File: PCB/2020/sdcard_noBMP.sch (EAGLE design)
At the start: 23 parts, among them J1 CONN_20X2NOSILK, J2 CONN_20X2NOSILK, J3 CONN_20X2NOSILK, J4 CONN_20X2NOSILK, X1 JST-XH-12-PIN-LONG-PAD, X2 JST-XH-06-PIN-LONG-PAD, X3 JST-XH-06-PIN-LONG-PAD, X4 JST-XH-12-PIN-LONG-PAD

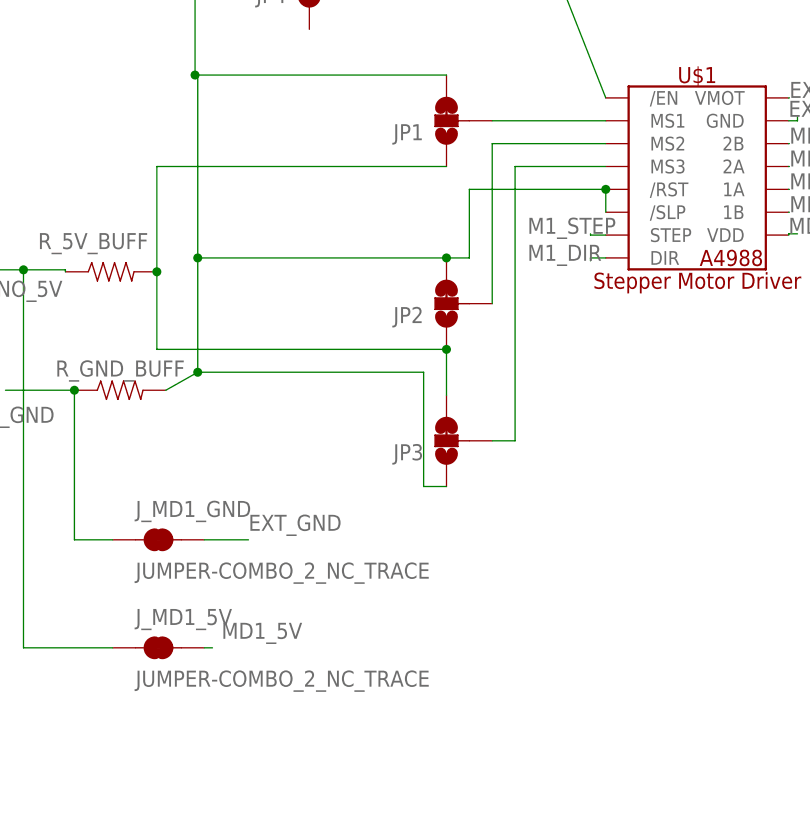
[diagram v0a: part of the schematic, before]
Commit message: PCB update
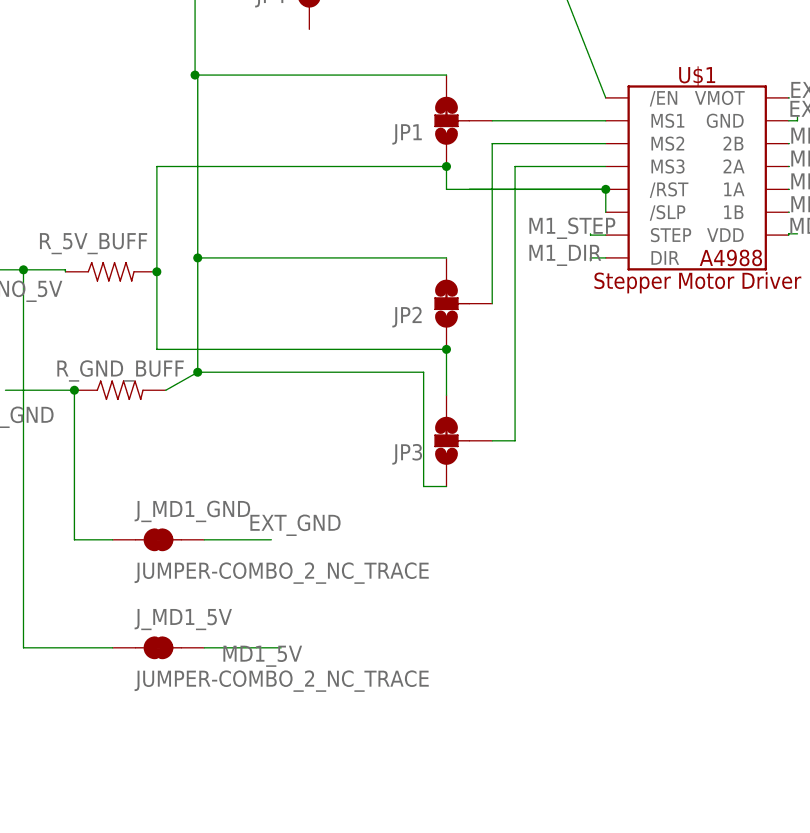
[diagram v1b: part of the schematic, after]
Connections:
- removed net N$9: JP1.1, JP2.1, JP3.3, R_5V_BUFF.2
- new net N$1: JP1.1, JP2.1, JP3.3, R_5V_BUFF.2, U$1./RST, U$1./SLP
- net N$14: no longer U$1./RST, U$1./SLP
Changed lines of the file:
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@@
 <?xml version="1.0" encoding="utf-8"?>
 <!DOCTYPE eagle SYSTEM "eagle.dtd">
-<eagle version="9.2.2">
+<eagle version="9.6.0">
 <drawing>
 <settings>
@@
 </segment>
 </net>
-<net name="N$9" class="0">
-<segment>
-<pinref part="R_5V_BUFF" gate="G$1" pin="2"/>
-<pinref part="JP1" gate="G$1" pin="1"/>
-<wire x1="105.82" y1="-33.22" x2="105.82" y2="-21.52" width="0.1524" layer="91"/>
-<wire x1="105.82" y1="-21.52" x2="138" y2="-21.52" width="0.1524" layer="91"/>
-<wire x1="105.82" y1="-33.22" x2="105.82" y2="-41.84" width="0.1524" layer="91"/>
-<junction x="105.82" y="-33.22"/>
-<pinref part="JP2" gate="G$1" pin="1"/>
-<wire x1="105.82" y1="-41.84" x2="138" y2="-41.84" width="0.1524" layer="91"/>
-<pinref part="JP3" gate="G$1" pin="3"/>
-<wire x1="138" y1="-41.84" x2="138" y2="-46.92" width="0.1524" layer="91"/>
-<junction x="138" y="-41.84"/>
-</segment>
-</net>
 <net name="N$14" class="0">
 <segment>
@@
 <pinref part="JP3" gate="G$1" pin="1"/>
 <wire x1="135.46" y1="-57.08" x2="138" y2="-57.08" width="0.1524" layer="91"/>
-<wire x1="138" y1="-31.68" x2="140.54" y2="-31.68" width="0.1524" layer="91"/>
-<wire x1="140.54" y1="-31.68" x2="140.54" y2="-24.06" width="0.1524" layer="91"/>
-<junction x="138" y="-31.68"/>
-<pinref part="U$1" gate="G$1" pin="/SLP"/>
-<pinref part="U$1" gate="G$1" pin="/RST"/>
-<wire x1="155.7" y1="-26.6" x2="155.7" y2="-24.06" width="0.1524" layer="91"/>
-<wire x1="140.54" y1="-24.06" x2="155.7" y2="-24.06" width="0.1524" layer="91"/>
-<junction x="155.7" y="-24.06"/>
 <pinref part="JP4" gate="G$1" pin="3"/>
 <wire x1="122.76" y1="3.88" x2="110.06" y2="3.88" width="0.1524" layer="91"/>
@@
 <segment>
 <pinref part="J_MD1_5V" gate="JP1" pin="2"/>
-<wire x1="112" y1="-75" x2="111.08" y2="-75" width="0.1524" layer="91"/>
-<label x="113" y="-74" size="1.778" layer="95"/>
+<wire x1="119.62" y1="-75" x2="111.08" y2="-75" width="0.1524" layer="91"/>
+<label x="113" y="-76.54" size="1.778" layer="95"/>
 </segment>
 <segment>
@@
 <segment>
 <pinref part="J_MD1_GND" gate="JP1" pin="2"/>
-<wire x1="111.08" y1="-63" x2="116" y2="-63" width="0.1524" layer="91"/>
+<wire x1="111.08" y1="-63" x2="118.54" y2="-63" width="0.1524" layer="91"/>
 <label x="116" y="-62" size="1.778" layer="95"/>
 </segment>
@@
 </segment>
 </net>
+<net name="N$1" class="0">
+<segment>
+<pinref part="U$1" gate="G$1" pin="/RST"/>
+<pinref part="U$1" gate="G$1" pin="/SLP"/>
+<wire x1="155.7" y1="-26.6" x2="155.7" y2="-24.06" width="0.1524" layer="91"/>
+<junction x="155.7" y="-24.06"/>
+<wire x1="140.54" y1="-24.06" x2="155.7" y2="-24.06" width="0.1524" layer="91"/>
+<pinref part="R_5V_BUFF" gate="G$1" pin="2"/>
+<pinref part="JP1" gate="G$1" pin="1"/>
+<wire x1="105.82" y1="-33.22" x2="105.82" y2="-21.52" width="0.1524" layer="91"/>
+<wire x1="105.82" y1="-21.52" x2="138" y2="-21.52" width="0.1524" layer="91"/>
+<wire x1="105.82" y1="-33.22" x2="105.82" y2="-41.84" width="0.1524" layer="91"/>
+<junction x="105.82" y="-33.22"/>
+<pinref part="JP2" gate="G$1" pin="1"/>
+<wire x1="105.82" y1="-41.84" x2="138" y2="-41.84" width="0.1524" layer="91"/>
+<pinref part="JP3" gate="G$1" pin="3"/>
+<wire x1="138" y1="-41.84" x2="138" y2="-46.92" width="0.1524" layer="91"/>
+<junction x="138" y="-41.84"/>
+<wire x1="155.7" y1="-24.06" x2="138" y2="-24.06" width="0.1524" layer="91"/>
+<wire x1="138" y1="-24.06" x2="138" y2="-21.52" width="0.1524" layer="91"/>
+<junction x="138" y="-21.52"/>
+</segment>
+</net>
